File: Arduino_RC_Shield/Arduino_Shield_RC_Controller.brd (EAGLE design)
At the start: 70 x 86 mm, 6 parts

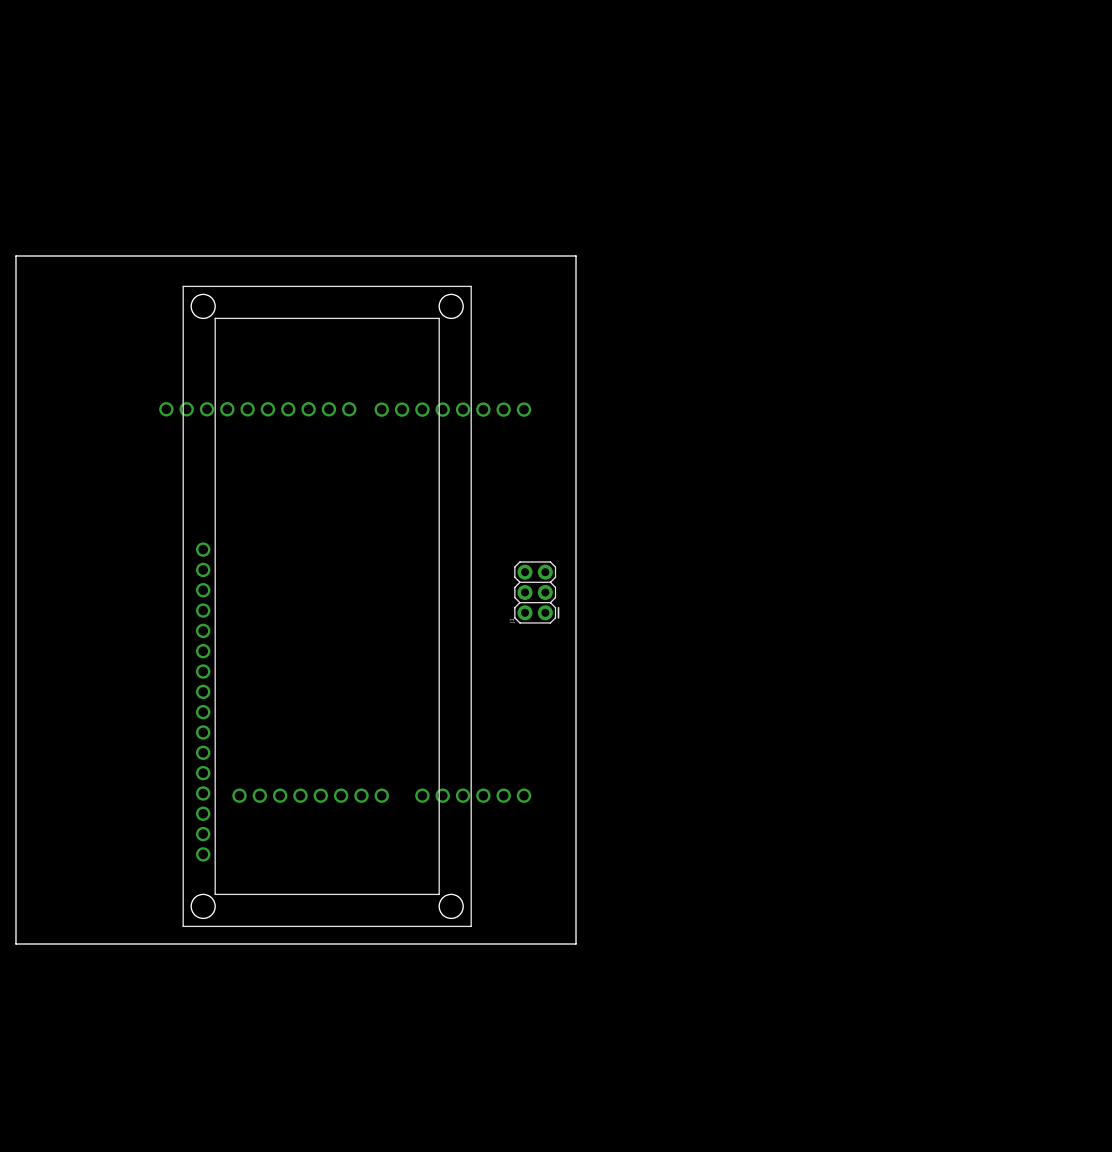
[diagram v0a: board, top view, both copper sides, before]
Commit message: update
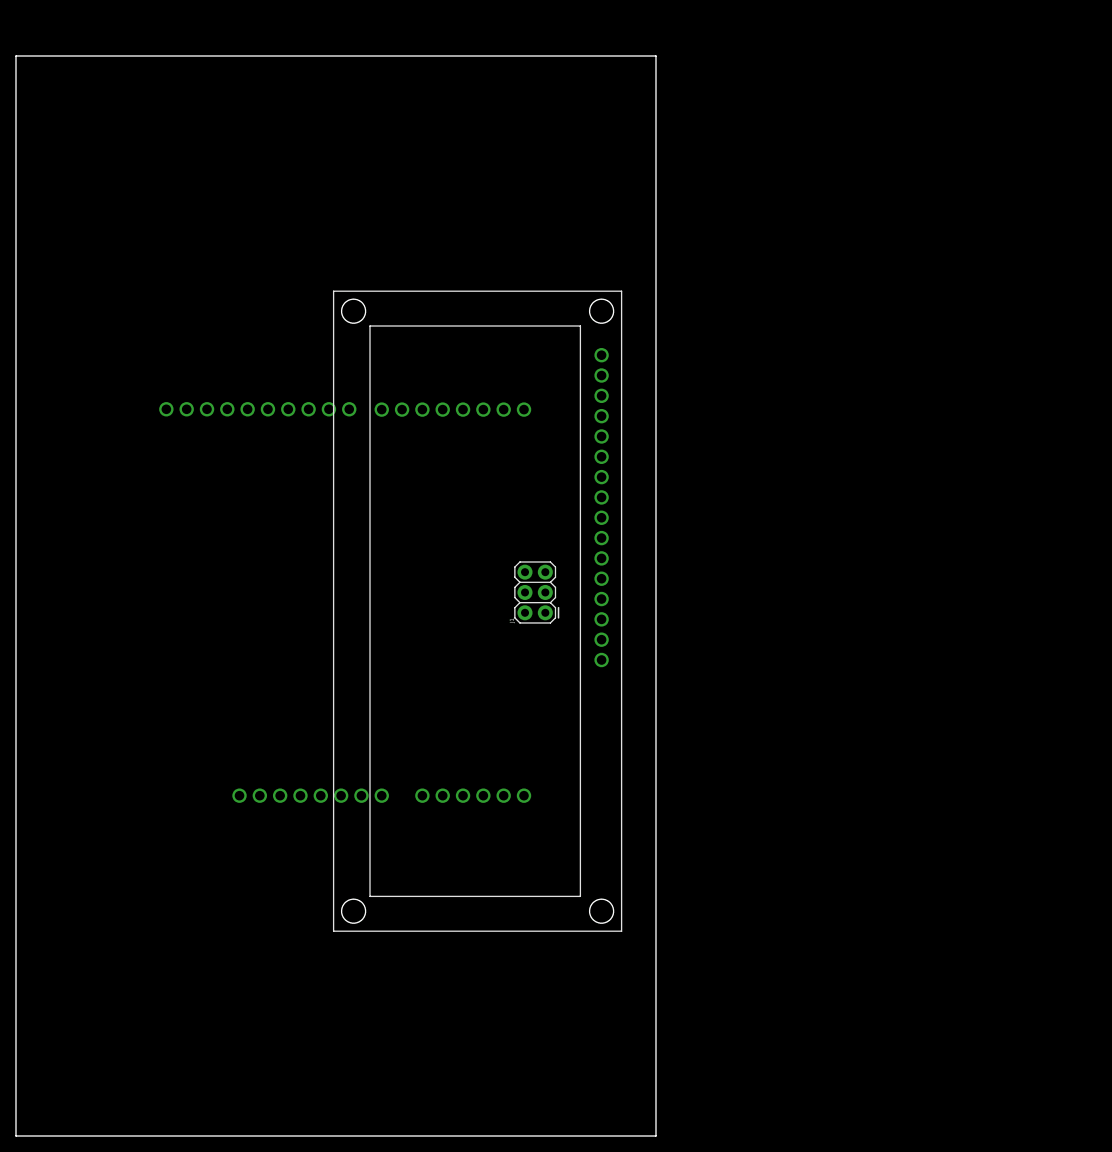
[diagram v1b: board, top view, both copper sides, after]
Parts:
- moved LCD1 18.8 mm to (39.7, 65.6)
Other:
- board size 70 x 86 mm -> 80 x 135 mm
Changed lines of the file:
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@@
 <board>
 <plain>
-<wire x1="0" y1="-16" x2="70" y2="-16" width="0" layer="20"/>
-<wire x1="70" y1="-16" x2="70" y2="70" width="0" layer="20"/>
-<wire x1="70" y1="70" x2="0" y2="70" width="0" layer="20"/>
-<wire x1="0" y1="70" x2="0" y2="-16" width="0" layer="20"/>
+<wire x1="0" y1="-40" x2="80" y2="-40" width="0" layer="20"/>
+<wire x1="80" y1="-40" x2="80" y2="95" width="0" layer="20"/>
+<wire x1="80" y1="95" x2="0" y2="95" width="0" layer="20"/>
+<wire x1="0" y1="95" x2="0" y2="-40" width="0" layer="20"/>
 </plain>
 <attributes>
@@
 </element>
 <element name="U$1" library="3D_MIG_Controller" package="HEADER_1_X_10_.1_INCH" value="1_X_10_HEADER_GENERIC_.1INCH" x="30.226" y="50.84" smashed="yes"/>
-<element name="LCD1" library="3D_MIG_Controller" package="ADM1602K" value="" x="20.9" y="66.2" smashed="yes" rot="R270"/>
+<element name="LCD1" library="3D_MIG_Controller" package="ADM1602K" value="" x="39.7" y="65.6" smashed="yes" rot="R270"/>
 </elements>
 <signals>

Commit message: Update
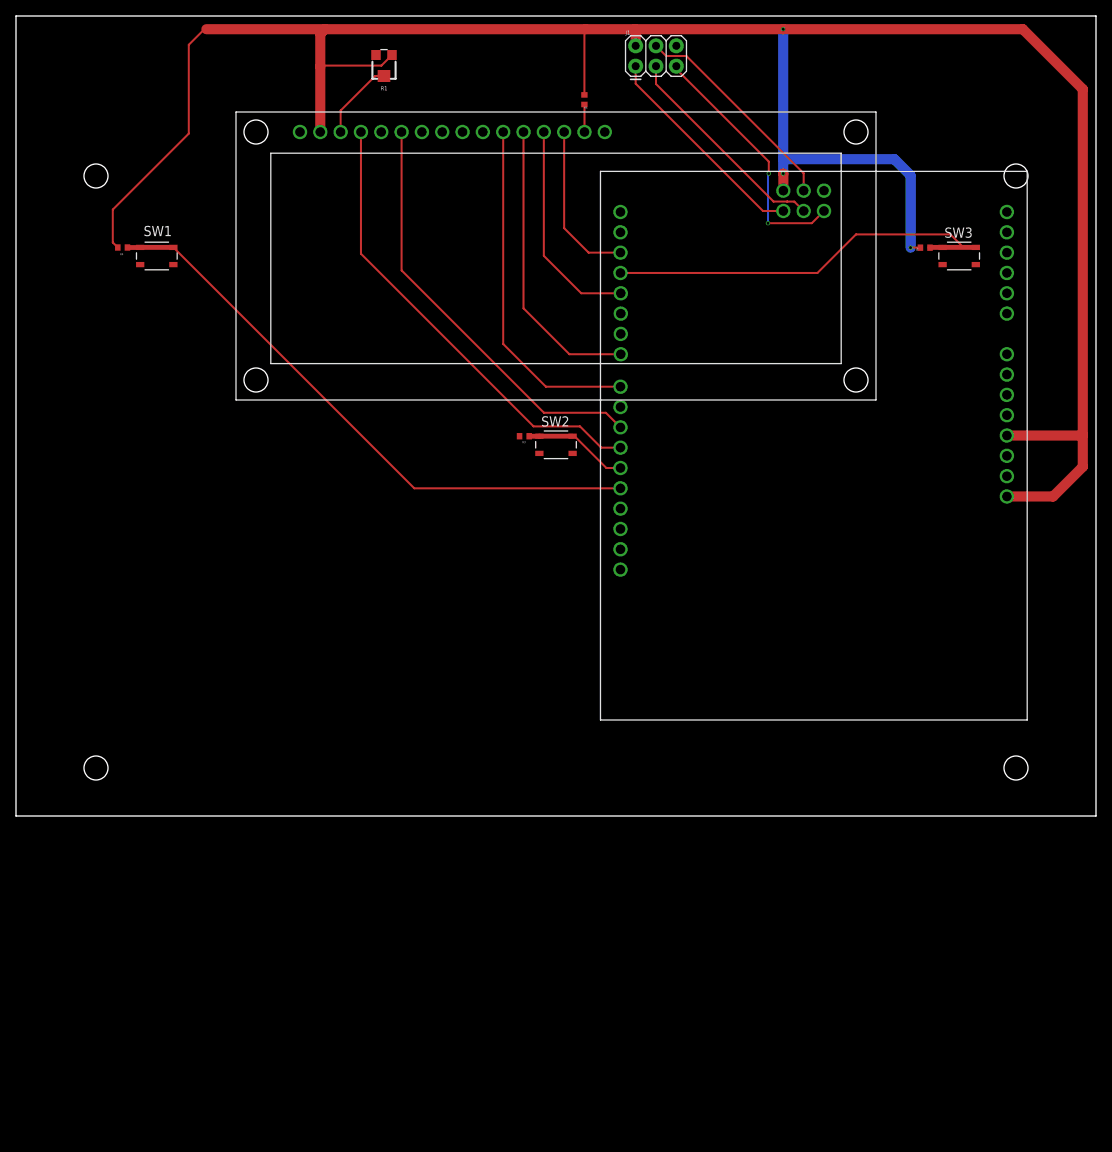
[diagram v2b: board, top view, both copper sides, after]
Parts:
- removed H1: (no value), 3D_MIG_Controller:HEADER_1_X_6_.1_INCH
- removed H2, H3: (no value), 3D_MIG_Controller:HEADER_1_X_8_.1_INCH
- removed U$1: 1_X_10_HEADER_GENERIC_.1INCH, 3D_MIG_Controller:HEADER_1_X_10_.1_INCH
- added AR1: (no value), 3D_MIG_Controller:ARDUINO_R3
- added R1: (no value), 3D_MIG_Controller:RTRIM3103
- added R2, R3, R4: 10K0, 3D_MIG_Controller:0402
- added R5: 470R0, 3D_MIG_Controller:0402
- added SW1, SW2, SW3: PTS810SJG250SMTRLFS, 3D_MIG_Controller:PTS810
- moved J1 68.7 mm to (80.0, 95.0), turned to 0 degrees
- moved LCD1 28.1 mm to (67.5, 70.0), turned to 0 degrees
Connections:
- new net A0: AR1.P30
- new net A1: AR1.P29
- new net A2: AR1.P28
- new net A3: AR1.P27
- new net A4: AR1.P26
- new net A5: AR1.P25
- new net AREF: AR1.P3
- new net CIPO: AR1.P19, J1.1
- new net COPI: AR1.P22, J1.4
- new net D4: AR1.P10, LCD1.P11
- new net D5: AR1.P11, LCD1.P12
- new net D6: AR1.P14, LCD1.P13
- new net D7: AR1.P16, LCD1.P14
- new net E: AR1.P8, LCD1.P6
- new net GND: AR1.P24, AR1.P32, AR1.P33, AR1.P4, J1.6, LCD1.P1, LCD1.P16, LCD1.P5, R1.3, SW1.3, SW1.4, SW2.3, SW2.4, SW3.3, SW3.4
- new net N$39: LCD1.P15, R5.P$1
- new net NC: AR1.P17, AR1.P18, AR1.P36, AR1.P37, AR1.P38, LCD1.P10, LCD1.P7, LCD1.P8, LCD1.P9
- new net PWM5: AR1.P13
- new net PWM6: AR1.P12
- new net PWM9: AR1.P9
- new net RESET: AR1.P23, J1.5
- new net RS: AR1.P7, LCD1.P4
- new net SCK: AR1.P21, J1.3
- new net SCL: AR1.P1
- new net SDA: AR1.P2
- new net SW1: AR1.P5, R4.P$2, SW1.1, SW1.2
- new net SW2: AR1.P6, R3.P$2, SW2.1, SW2.2
- new net SW3: AR1.P15, R2.P$2, SW3.1, SW3.2
- new net V0: LCD1.P3, R1.2
- new net VDD: AR1.P35
- new net VDD5: AR1.P20, AR1.P31, AR1.P34, J1.2, LCD1.P2, R1.1, R2.P$1, R3.P$1, R4.P$1, R5.P$2
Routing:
- net VDD5: track 0.00 -> 293.1 mm, vias 0 -> 3
- net SW1: track 0.00 -> 74.1 mm
- net RS: track 0.00 -> 57.7 mm
- net SW3: track 0.00 -> 52.8 mm
- net E: track 0.00 -> 52.8 mm
- net D4: track 0.00 -> 43.4 mm
- net D5: track 0.00 -> 36.6 mm
- net RESET: track 0.00 -> 32.1 mm, vias 0 -> 2
- net SCK: track 0.00 -> 27.3 mm
- net CIPO: track 0.00 -> 27.2 mm
- net COPI: track 0.00 -> 27.2 mm
- net D6: track 0.00 -> 27.0 mm
- net D7: track 0.00 -> 20.3 mm
- net SW2: track 0.00 -> 13.1 mm
- net V0: track 0.00 -> 9.89 mm
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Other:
- board size 80 x 135 mm -> 135 x 100 mm
